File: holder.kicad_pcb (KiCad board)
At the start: 2 copper layers, 58 x 88 mm, 25 parts

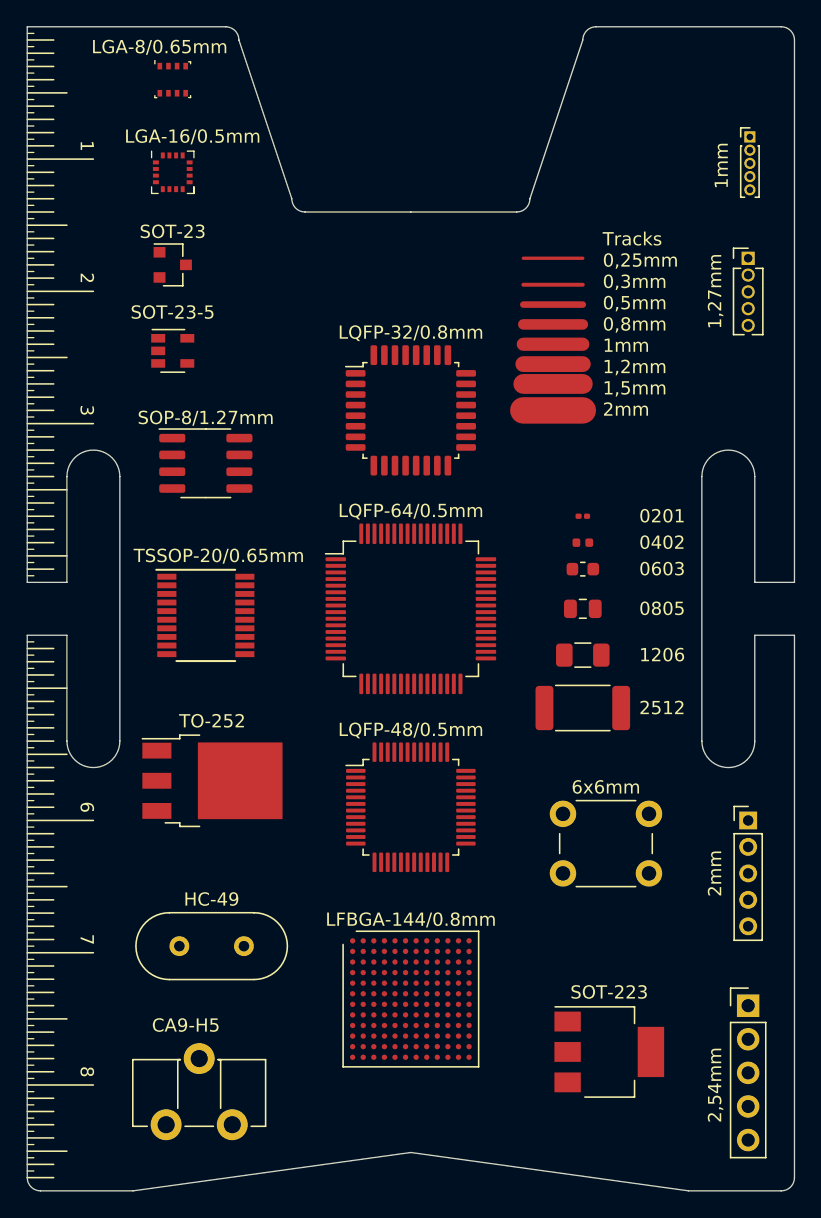
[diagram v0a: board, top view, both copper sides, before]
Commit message: added field
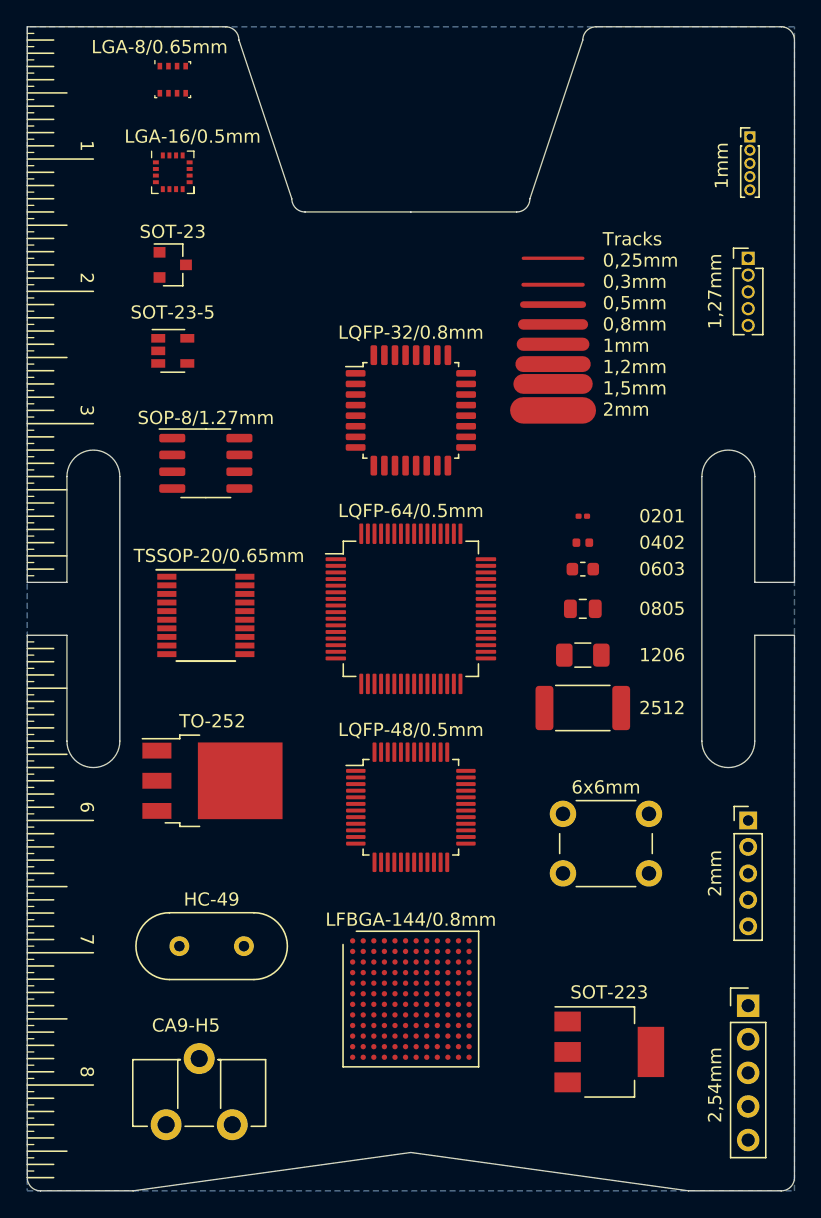
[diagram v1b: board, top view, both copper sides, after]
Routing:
- added copper zone on B.Cu, net (none)
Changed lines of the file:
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@@
   )
   (setup
-    (last_trace_width 2)
+    (last_trace_width 0.25)
     (user_trace_width 0.3)
     (user_trace_width 0.5)
@@
   (segment (start 197.5 87) (end 202 87) (width 1.5) (layer F.Cu) (net 0))
   (segment (start 197.5 89) (end 202 89) (width 2) (layer F.Cu) (net 0))
+  (zone (net 0) (net_name "") (layer B.Cu) (hatch edge 0.508)
+    (connect_pads (clearance 0.508))
+    (min_thickness 0.254)
+    (fill yes (arc_segments 32) (thermal_gap 0.508) (thermal_bridge_width 0.508))
+    (polygon
+      (pts
+        (xy 160 60) (xy 160 148) (xy 218 148) (xy 218 60)
+      )
+    )
+  )
 )
